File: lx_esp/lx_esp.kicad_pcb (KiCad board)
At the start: 4 copper layers, 74 x 24 mm, 26 parts, among them J1 Conn_01x02, J2 200LX_02X05, Q1 Dual_Nch_MOSFET, SW1 SW_Push, SW2 SW_SPDT, U1 LTC4365, U2 XC6210, U3 ESP-12F, U4 TRS3238E

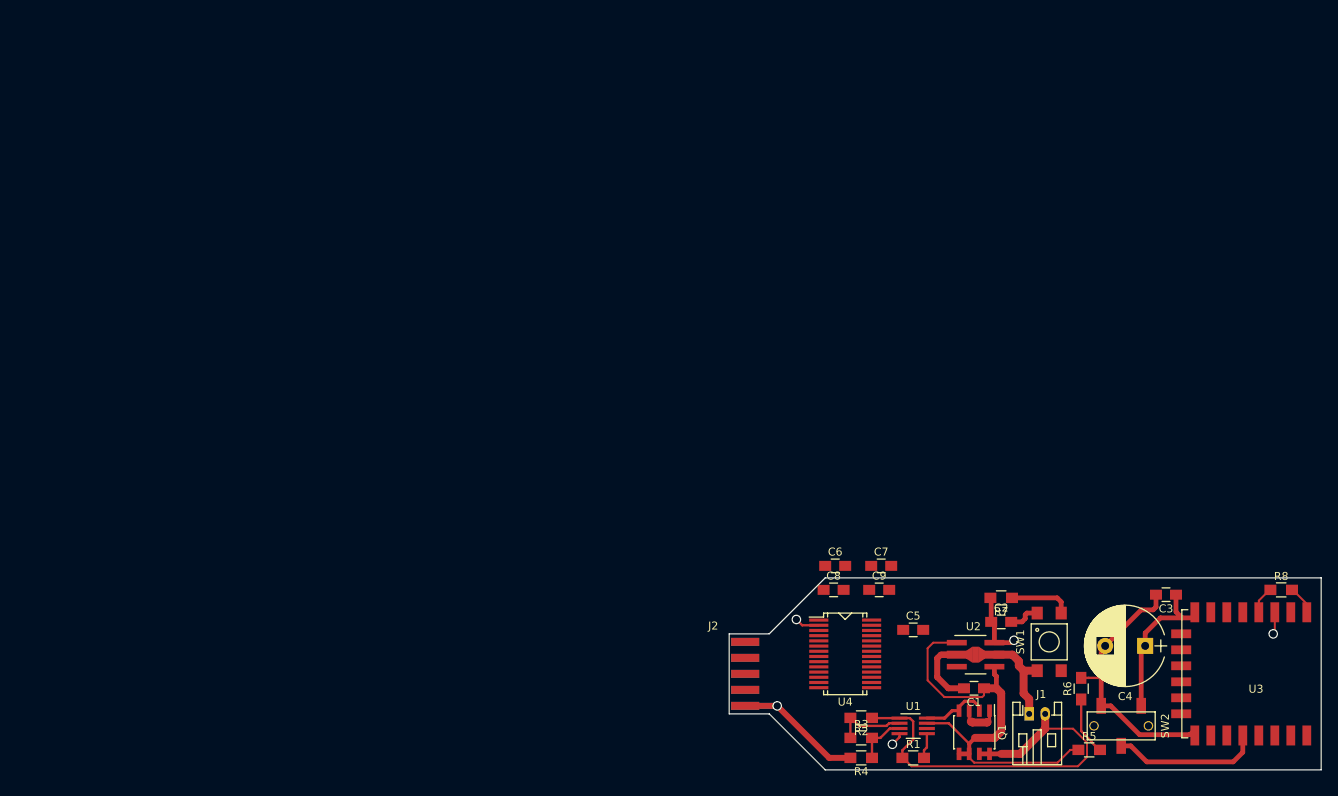
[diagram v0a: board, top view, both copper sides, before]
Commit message: more pcb layout
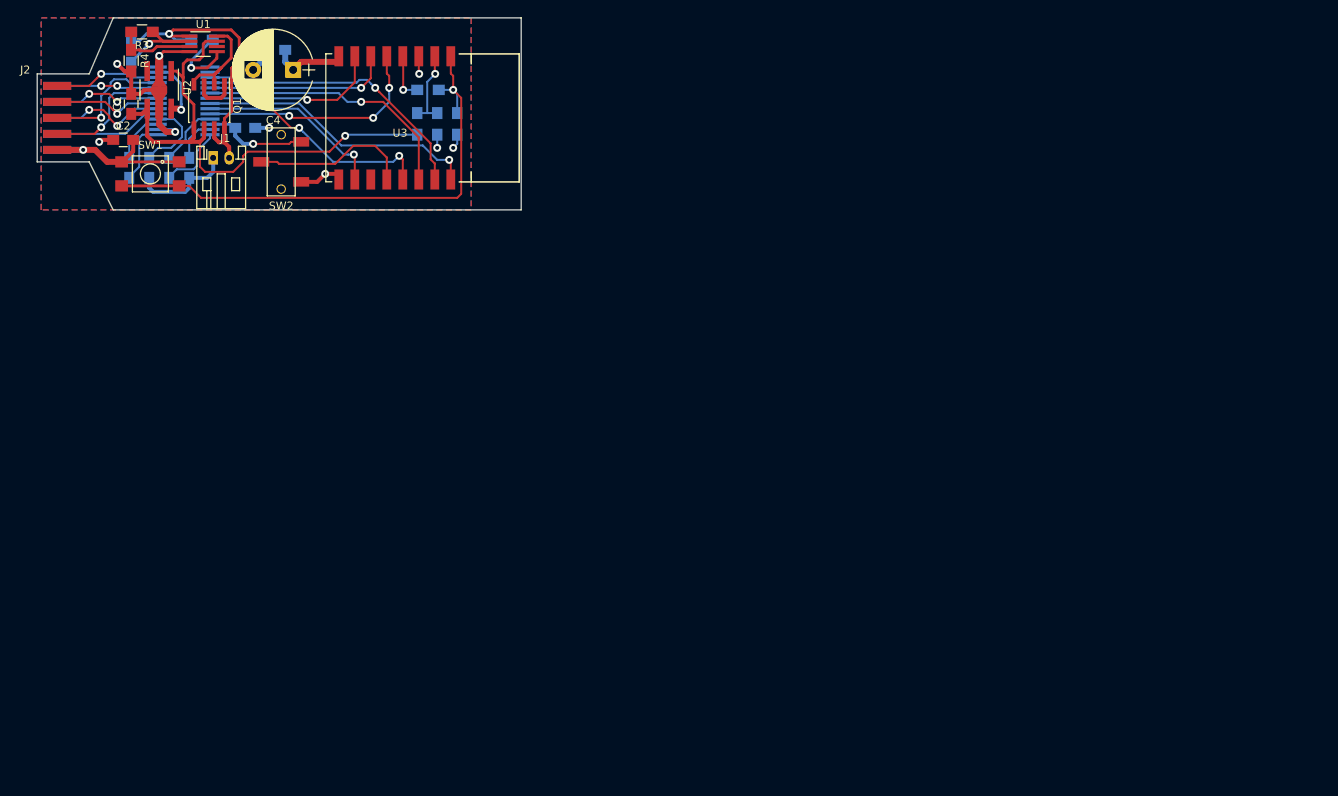
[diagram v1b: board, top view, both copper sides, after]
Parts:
- C3, C5, C6, C7, C8, C9, R1, R2, R5, R6, R7, R8, U4: moved to B.Cu
- U3: footprint ESP8266:ESP-12E_SMD -> ssop_20:ESP-12E_SMD_hax
- moved C3 130.5 mm to (59.2, 27.5)
- moved C4 128.6 mm to (61.5, 30.0)
- moved C1 128.2 mm to (41.2, 34.2), turned to 90 degrees
- moved U3 127.6 mm to (81.2, 29.0)
- moved SW1 126.7 mm to (43.6, 43.0), turned to 180 degrees
- moved SW2 126.5 mm to (60.0, 41.5), turned to 90 degrees
- moved R1 126.3 mm to (50.1, 26.2)
- moved R4 126.2 mm to (41.2, 28.9), turned to 270 degrees
- moved R3 126.0 mm to (42.6, 25.2), turned to 180 degrees
- moved C2 125.2 mm to (40.2, 38.8)
- moved U2 124.1 mm to (44.8, 32.5), turned to 270 degrees
- moved R8 123.6 mm to (78.3, 32.5)
- moved Q1 123.6 mm to (51.0, 34.5)
- moved R2 123.5 mm to (41.2, 27.8), turned to 270 degrees
- moved J1 123.4 mm to (51.5, 41.0)
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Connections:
- U1 pad 6: Net-(U1-Pad6) -> (no net)
- U2 pad 3: Net-(U2-Pad3) -> (no net)
- U3 pad 11: Net-(U3-Pad11) -> (no net)
- U3 pad 17: Net-(U3-Pad17) -> (no net)
- U3 pad 18: Net-(U3-Pad18) -> (no net)
- U3 pad 19: Net-(U3-Pad19) -> (no net)
- U3 pad 20: Net-(U3-Pad20) -> (no net)
- U3 pad 21: Net-(U3-Pad21) -> (no net)
- U3 pad 22: Net-(U3-Pad22) -> (no net)
- U4 pad 10: Net-(J2-Pad8) -> Net-(J2-Pad6)
- U4 pad 12: Net-(J2-Pad9) -> Net-(J2-Pad1)
- U4 pad 14: Net-(U4-Pad14) -> (no net)
- U4 pad 15: Net-(U4-Pad15) -> (no net)
- U4 pad 16: Net-(U4-Pad16) -> (no net)
- U4 pad 17: /RI -> /CD
- U4 pad 19: /UART0_RTS -> /DSR
- U4 pad 22: /DSR -> /UART0_TXD
- U4 pad 23: /UART0_TXD -> /UART0_RTS
- U4 pad 24: /CD -> /RI
- U4 pad 5: Net-(J2-Pad1) -> Net-(J2-Pad9)
- U4 pad 6: Net-(J2-Pad2) -> Net-(J2-Pad8)
- U4 pad 7: Net-(J2-Pad6) -> Net-(J2-Pad2)
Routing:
- net Net-(R7-Pad1): track 12.1 -> 65.2 mm, vias 0 -> 1
- net /UART0_RXD: track 0.00 -> 35.0 mm, vias 0 -> 1
- net /UART0_TXD: track 0.00 -> 34.7 mm, vias 0 -> 1
- net /DTR: track 0.00 -> 32.9 mm, vias 0 -> 1
- net /CD: track 0.00 -> 30.9 mm, vias 0 -> 3
- net /RI: track 0.00 -> 28.6 mm, vias 0 -> 3
- net /UART0_RTS: track 0.00 -> 22.8 mm, vias 0 -> 1
- net /DSR: track 0.00 -> 22.7 mm, vias 0 -> 1
- net /UART0_CTS: track 0.00 -> 21.6 mm, vias 0 -> 1
- net Net-(J2-Pad3): track 0.00 -> 16.5 mm, vias 0 -> 1
- net Net-(J2-Pad4): track 0.00 -> 16.2 mm, vias 0 -> 1
- net Net-(J2-Pad8): track 0.00 -> 14.8 mm, vias 0 -> 2
- net Net-(J1-Pad2): track 53.6 -> 39.0 mm, vias 0 -> 1
- net Net-(J2-Pad2): track 0.00 -> 13.7 mm, vias 0 -> 1
- net Net-(J2-Pad9): track 0.00 -> 13.5 mm
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- added copper zone on B.Cu, net GND
- added copper zone on F.Cu, net GND
- added copper zone on In2.Cu, net GND
- added copper zone on In1.Cu, net VCC
- removed copper zone on In1.Cu, net GND
- removed copper zone on In2.Cu, net VCC
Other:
- board size 74 x 24 mm -> 60.5 x 24 mm
- net class Default: via_dia 1.2 -> 1; via_drill 0.9 -> 0.5

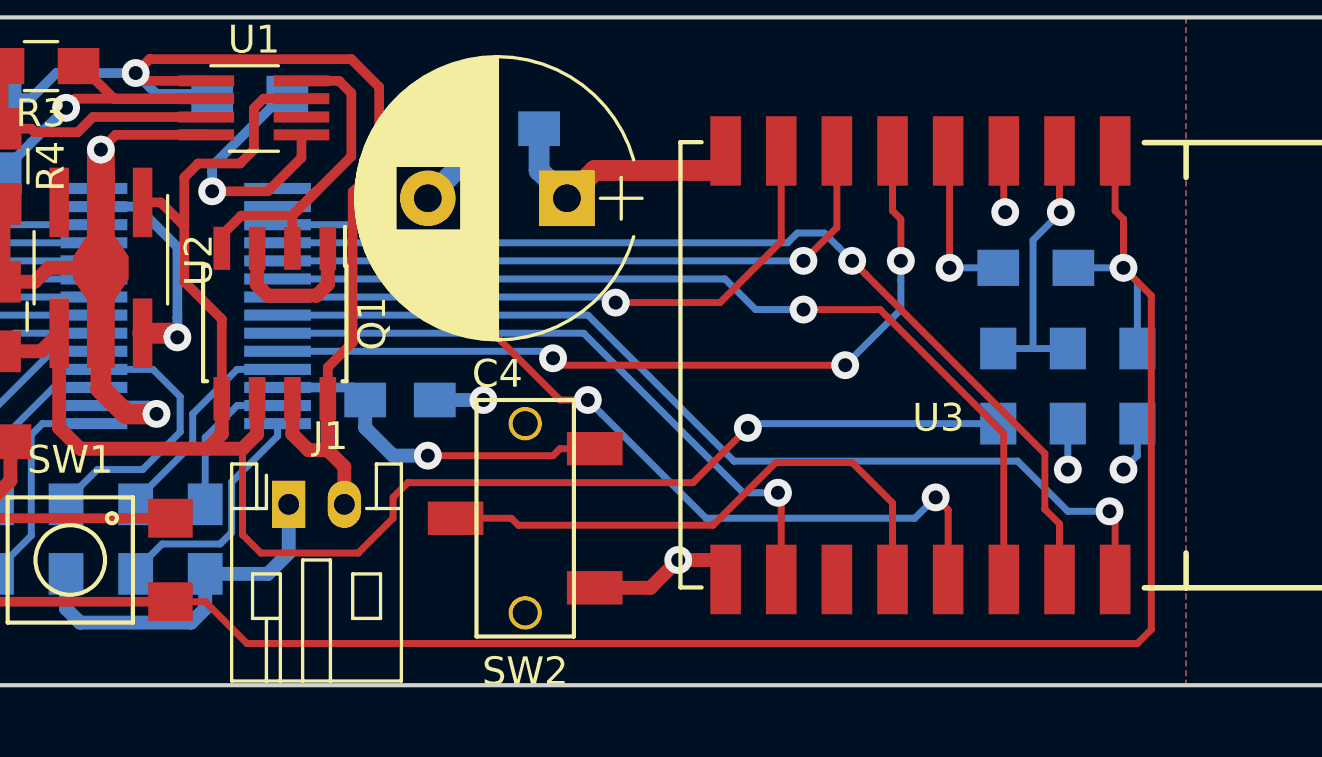
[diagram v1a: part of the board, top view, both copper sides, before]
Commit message: pcb tweaks
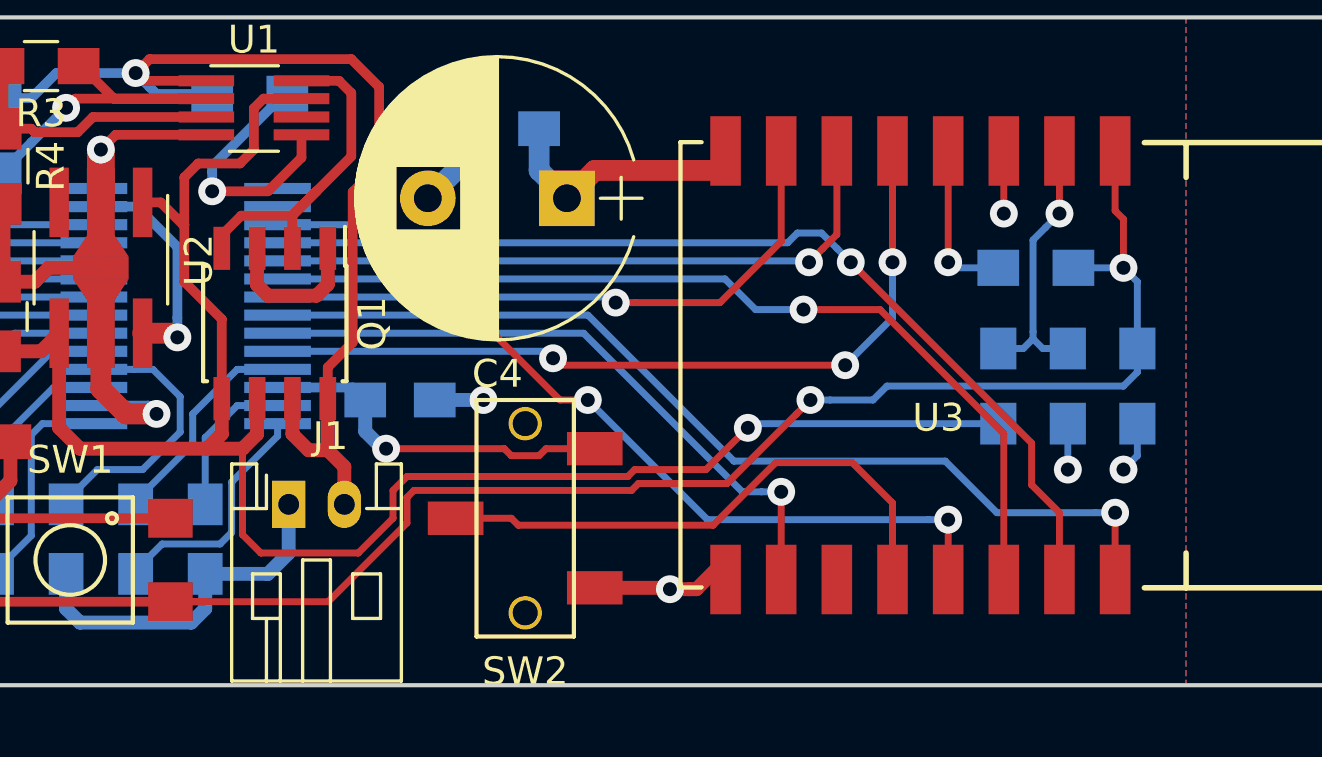
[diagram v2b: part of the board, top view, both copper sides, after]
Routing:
- net Net-(R7-Pad1): track 65.2 -> 56.9 mm, vias 1 -> 2
- net /CD: track 30.9 -> 30.1 mm
